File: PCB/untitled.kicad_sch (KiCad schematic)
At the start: 5 parts, among them J1 Conn_01x02, Q1 IRLML0030

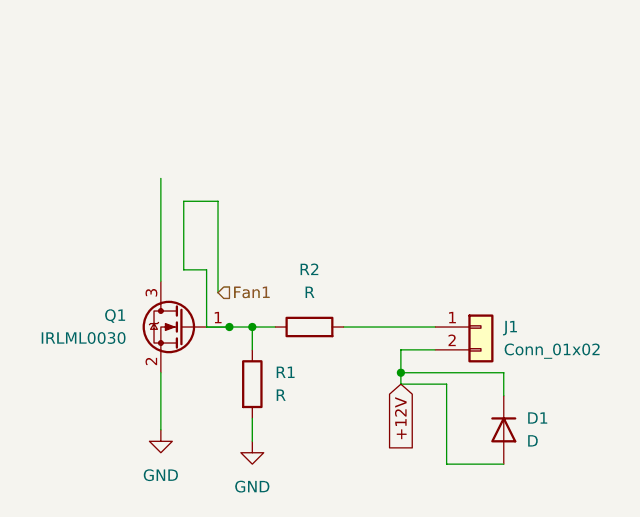
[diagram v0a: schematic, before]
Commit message: finished PCB
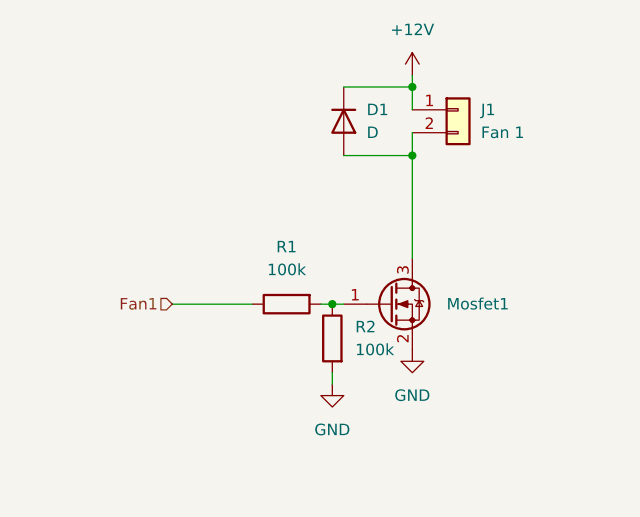
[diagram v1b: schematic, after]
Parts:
- removed Q1: IRLML0030, Package_TO_SOT_SMD:SOT-23, symbol Transistor_FET:IRLML0030
- added Mosfet1: IRLML0030, Package_TO_SOT_SMD:SOT-23, symbol Transistor_FET:IRLML0030
- J1: value Conn_01x02 -> Fan 1
- R1, R2: value R -> 100k
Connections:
- net +12V: now also J1.1 (Pin_1); no longer D1.2 (A), J1.2 (Pin_2)
- net Fan1: no longer R2.1
- net GND: now also R2.2, Mosfet1.2 (S); no longer R1.2
- new net: Mosfet1.1 (G), R1.2, R2.1
- new net: D1.2 (A), J1.2 (Pin_2), Mosfet1.3 (D)
